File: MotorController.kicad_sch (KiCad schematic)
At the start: 131 parts, among them IC1 ft234xd, IC2 A3921KLPTR-T, IC3 A3921KLPTR-T, J1 SH, J10 PA, J11 XT30, J2 USB_B_Micro, J3 XA, J4 XA, J5 3020-10-0300-00, J6 SH, J7 SH, J8 3020-10-0300-00, J9 XA, Q1 GSFQ6806, Q2 GSFQ6806, Q3 GSFQ6806, Q4 SFS9Z34, Q5 GSFQ6806, Q6 SFS9Z34, SW2 BLACK, SW3 BLACK, SW4 2MS1-T1-B4-VS2-Q-E-S, SW5 RED, U1 LXES11D, U2 STM32F303K8Tx, U3 TJA1441AT, U4 TPSM13604HNDWR, U5 LMZ12002EXT, Y1 32M

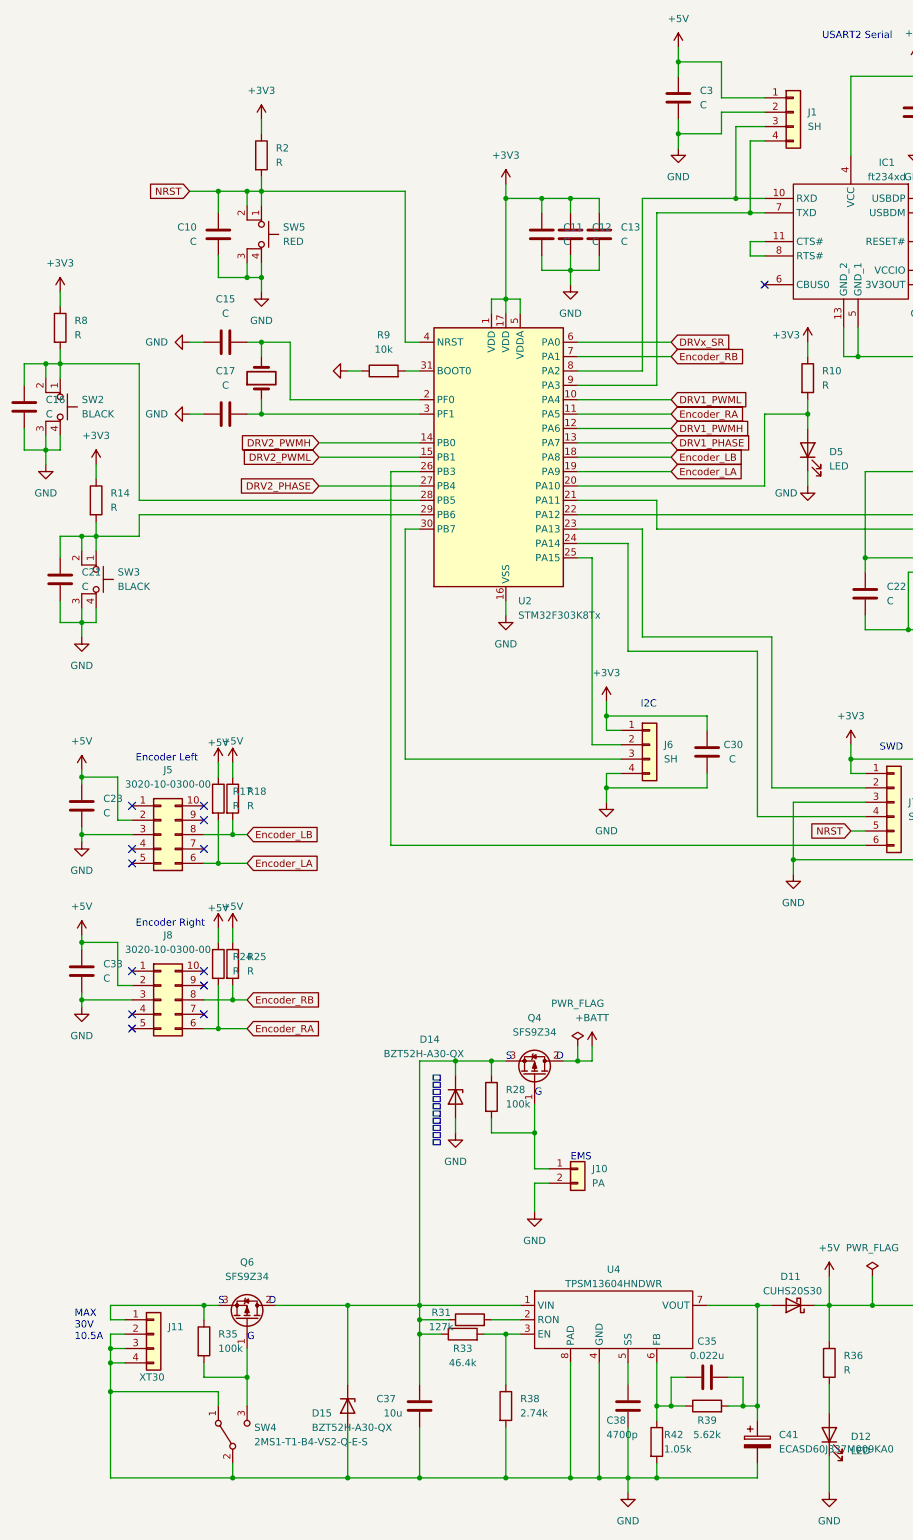
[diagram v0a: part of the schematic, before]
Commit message: Z 実装
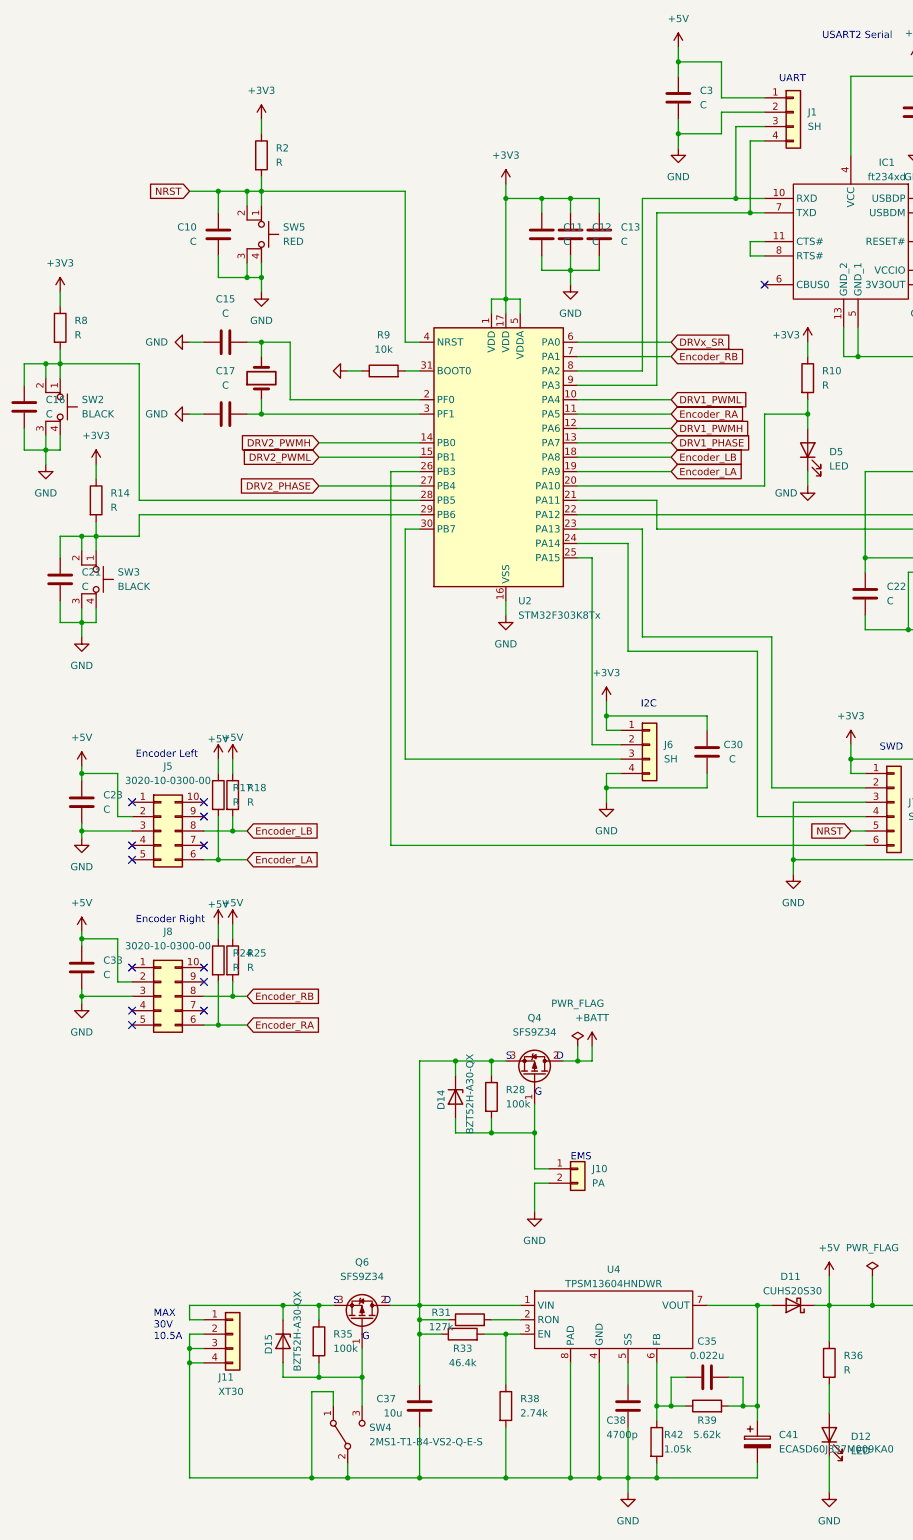
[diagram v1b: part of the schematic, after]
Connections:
- net GND: no longer D14.2 (A), D15.2 (A)
- net at J10.1 (Pin_1), Q4.1 (G), R28.2: now also D14.2 (A)
- net at C37.1, D14.1 (K), Q4.3 (S)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: no longer D15.1 (K)
- net at Q6.1 (G), R35.2, SW4.3 (C): now also D15.2 (A)
- net at J11.1 (Pin_1), Q6.3 (S), R35.1: now also D15.1 (K)
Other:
- note added: "UART"
- note removed: "ここじゃないのか疑問"
- moved on the sheet: C23, C33, D15, J11, J5, J8, Q6, R17, R18, R24, R25, R35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

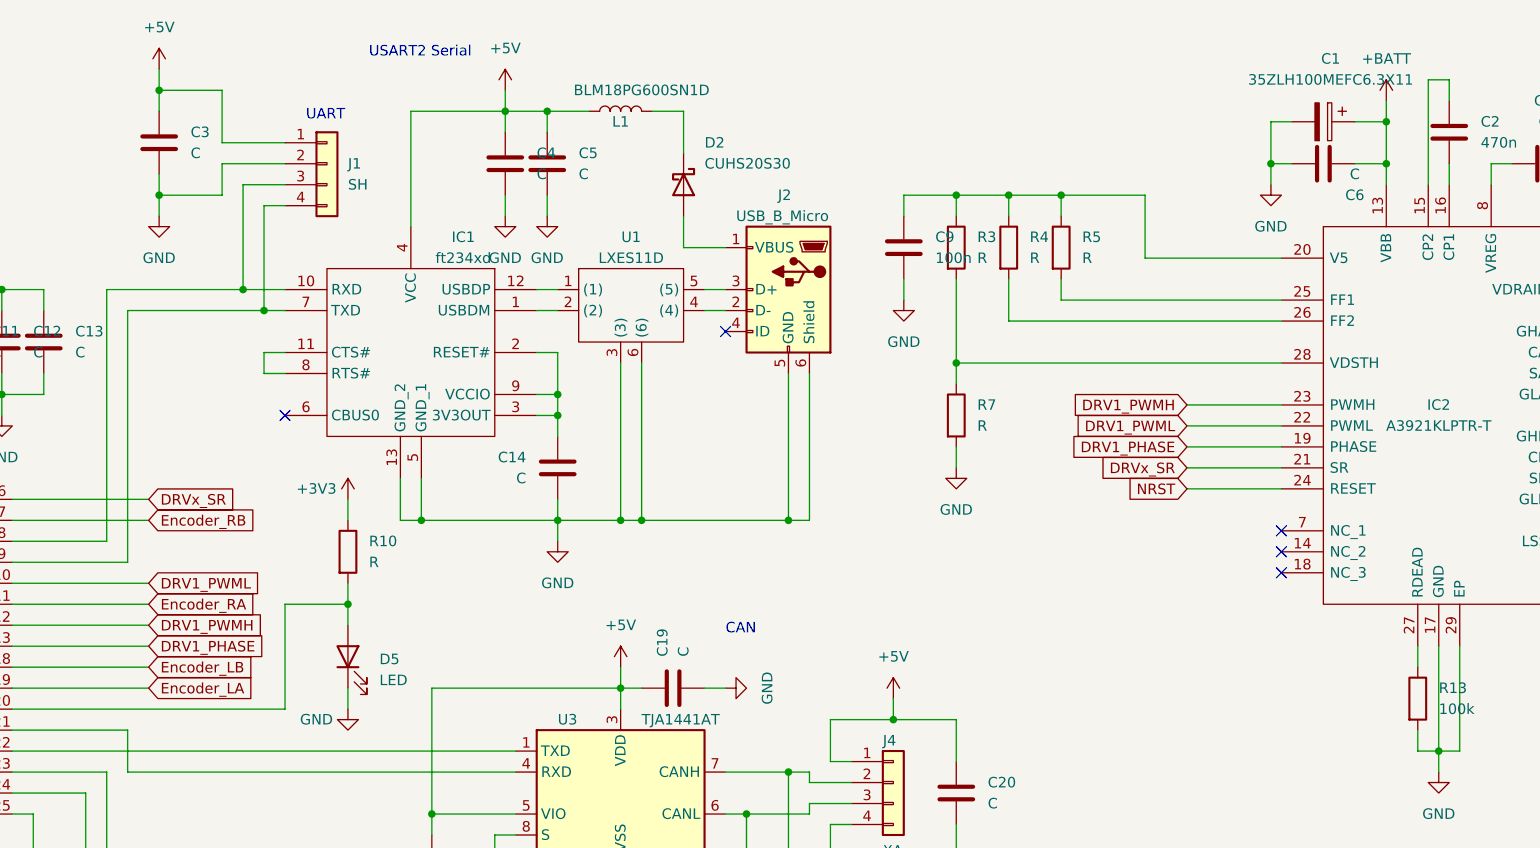
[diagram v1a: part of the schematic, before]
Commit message: CPU CAN MD DCDC の位置感決めた あとは UI
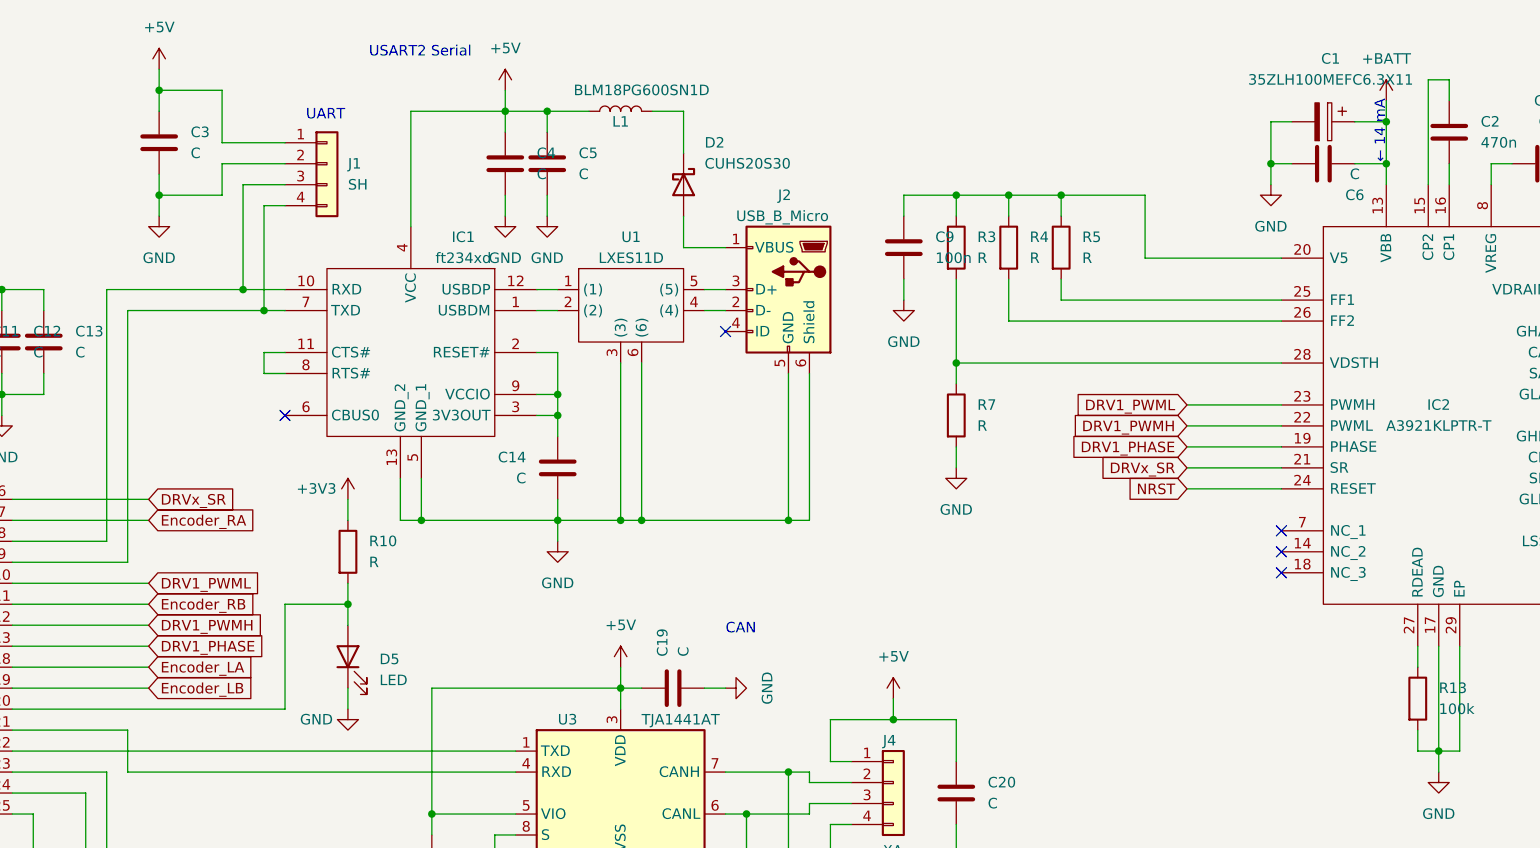
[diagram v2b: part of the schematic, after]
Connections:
- net DRV1_PWMH: now also IC2.22 (PWML); no longer IC2.23 (PWMH)
- net DRV1_PWML: now also IC2.23 (PWMH); no longer IC2.22 (PWML)
- net Encoder_LA: now also U2.18 (PA8); no longer U2.19 (PA9)
- net Encoder_LB: now also U2.19 (PA9); no longer U2.18 (PA8)
- net Encoder_RA: now also U2.7 (PA1); no longer U2.11 (PA5)
- net Encoder_RB: now also U2.11 (PA5); no longer U2.7 (PA1)
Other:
- note added: "← 14 mA"
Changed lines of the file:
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@@
     (effects (font (size 1.27 1.27)) (justify right bottom))
+  )
+  (text "← 14 mA" (at 279.4 33.02 90)
+    (effects (font (size 1.27 1.27)) (justify left bottom))
   )
   (text "SWD" (at 166.37 146.05 0)
@@
     )
   )
-  (global_label "Encoder_RA" (shape input) (at 129.54 86.36 0) (fields_autoplaced)
+  (global_label "Encoder_RA" (shape input) (at 129.54 76.2 0) (fields_autoplaced)
     (effects (font (size 1.27 1.27)) (justify left))
-    (property "Intersheetrefs" "${INTERSHEET_REFS}" (at 143.4108 86.36 0)
+    (property "Intersheetrefs" "${INTERSHEET_REFS}" (at 143.4108 76.2 0)
       (effects (font (size 1.27 1.27)) (justify left) hide)
     )
@@
     )
   )
-  (global_label "Encoder_RB" (shape input) (at 129.54 76.2 0) (fields_autoplaced)
+  (global_label "Encoder_RB" (shape input) (at 129.54 86.36 0) (fields_autoplaced)
     (effects (font (size 1.27 1.27)) (justify left))
-    (property "Intersheetrefs" "${INTERSHEET_REFS}" (at 143.5922 76.2 0)
+    (property "Intersheetrefs" "${INTERSHEET_REFS}" (at 143.5922 86.36 0)
       (effects (font (size 1.27 1.27)) (justify left) hide)
     )
@@
     )
   )
-  (global_label "Encoder_LA" (shape input) (at 129.54 96.52 0) (fields_autoplaced)
+  (global_label "Encoder_LA" (shape input) (at 129.54 93.98 0) (fields_autoplaced)
     (effects (font (size 1.27 1.27)) (justify left))
-    (property "Intersheetrefs" "${INTERSHEET_REFS}" (at 143.1689 96.52 0)
+    (property "Intersheetrefs" "${INTERSHEET_REFS}" (at 143.1689 93.98 0)
       (effects (font (size 1.27 1.27)) (justify left) hide)
     )
@@
     )
   )
-  (global_label "DRV1_PWML" (shape input) (at 255.27 64.77 180) (fields_autoplaced)
+  (global_label "DRV1_PWML" (shape input) (at 255.27 62.23 180) (fields_autoplaced)
     (effects (font (size 1.27 1.27)) (justify right))
-    (property "Intersheetrefs" "${INTERSHEET_REFS}" (at 241.2782 64.77 0)
+    (property "Intersheetrefs" "${INTERSHEET_REFS}" (at 241.2782 62.23 0)
       (effects (font (size 1.27 1.27)) (justify right) hide)
     )
@@
     )
   )
-  (global_label "DRV1_PWMH" (shape input) (at 255.27 62.23 180) (fields_autoplaced)
+  (global_label "DRV1_PWMH" (shape input) (at 255.27 64.77 180) (fields_autoplaced)
     (effects (font (size 1.27 1.27)) (justify right))
-    (property "Intersheetrefs" "${INTERSHEET_REFS}" (at 240.9758 62.23 0)
+    (property "Intersheetrefs" "${INTERSHEET_REFS}" (at 240.9758 64.77 0)
       (effects (font (size 1.27 1.27)) (justify right) hide)
     )
@@
     )
   )
-  (global_label "Encoder_LB" (shape input) (at 129.54 93.98 0) (fields_autoplaced)
+  (global_label "Encoder_LB" (shape input) (at 129.54 96.52 0) (fields_autoplaced)
     (effects (font (size 1.27 1.27)) (justify left))
-    (property "Intersheetrefs" "${INTERSHEET_REFS}" (at 143.3503 93.98 0)
+    (property "Intersheetrefs" "${INTERSHEET_REFS}" (at 143.3503 96.52 0)
       (effects (font (size 1.27 1.27)) (justify left) hide)
     )
